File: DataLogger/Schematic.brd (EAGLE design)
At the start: 78.4 x 66 mm, 29 parts, among them J1 DCJ0202, Q1 IRLML5203, U1 ATMEGA328P-AU

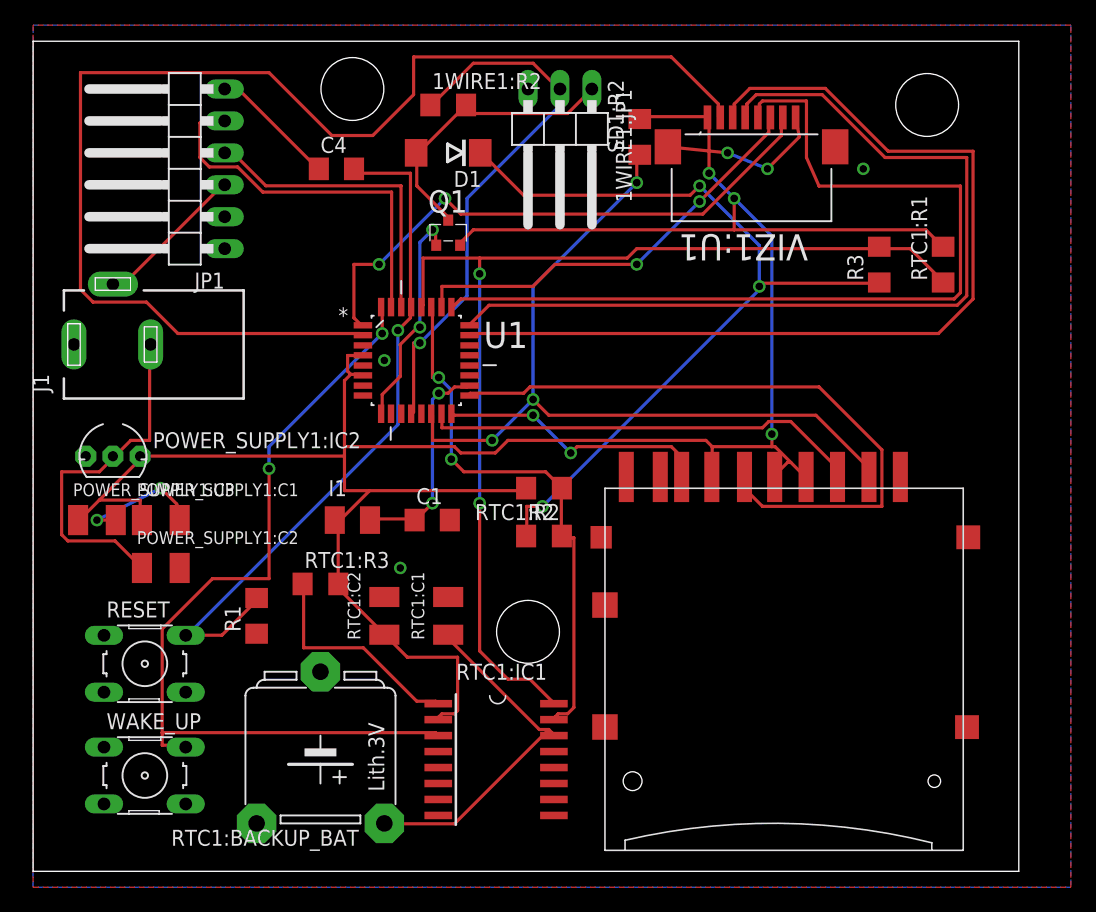
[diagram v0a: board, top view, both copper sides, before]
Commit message: Improvements
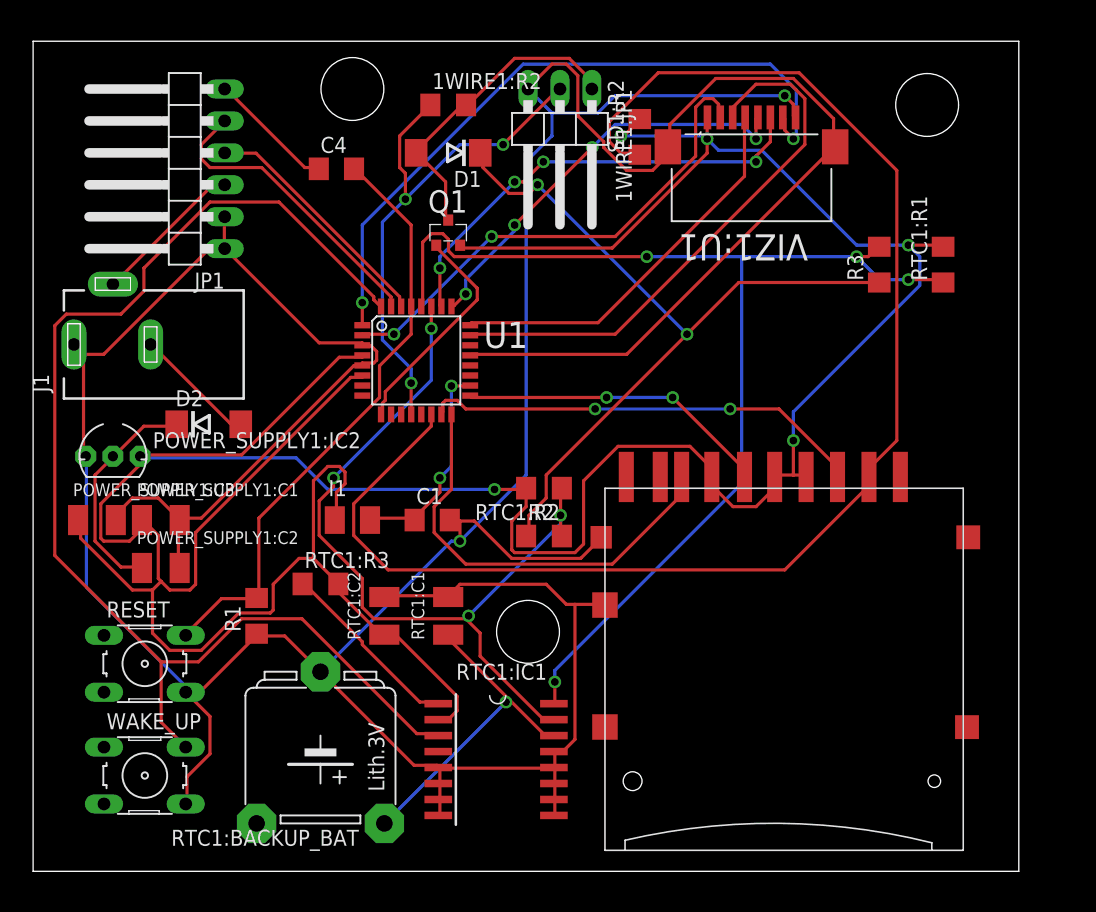
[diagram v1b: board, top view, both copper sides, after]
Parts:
- added D2: (no value), diode:DO214AA
- U1: device atmel-atmeg328PU:QFP80P900X900X120-32N -> Arduino Dev Parts:TQFP32-08
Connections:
- net CS renamed D10
- net MISO renamed D12
- net MOSI renamed D11
- net N$1 renamed D5
- net N$10 renamed A4
- net N$15 renamed D2
- net N$16 renamed D8
- net N$18 renamed D4
- net N$3 renamed A0
- net N$4 renamed A1
- net N$5 renamed A2
- net N$6 renamed A3
- net N$8 renamed D3
- net N$9 renamed A5
- net SCK renamed D13
- removed net ADC6: U1.19
- removed net ADC7: U1.22
- new net N$1: D2.A, J1.3
- net N$2: now also D2.C; no longer J1.3
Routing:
- net GND: track 23.6 -> 351.4 mm, vias 7 -> 2
- net VCC: track 202.4 -> 280.6 mm, vias 3 -> 5
- net D4: track 101.1 -> 39.8 mm, vias 0 -> 2
- net D10: track 64.2 -> 115.2 mm, vias 3 -> 0
- net A1: track 72.6 -> 31.5 mm
- net A2: track 72.6 -> 33.4 mm, vias 0 -> 4
- net A0: track 75.8 -> 44.3 mm
- net D2: track 68.8 -> 99.8 mm, vias 2 -> 0
- net D13: track 52.2 -> 24.9 mm, vias 0 -> 2
- net A4: track 43.2 -> 64.3 mm, vias 2 -> 4
- net D12: track 21.7 -> 34.4 mm, vias 2 -> 0
- net N$2: track 28.2 -> 18.1 mm
- net N$1: track 0.00 -> 9.77 mm
- net D3: track 46.0 -> 54.7 mm
- net RESET: track 55.8 -> 48.0 mm, vias 1 -> 0
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- removed copper zone on layer 1, net GND
- removed copper zone on layer 16, net GND
